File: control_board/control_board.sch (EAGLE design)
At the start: 86 parts

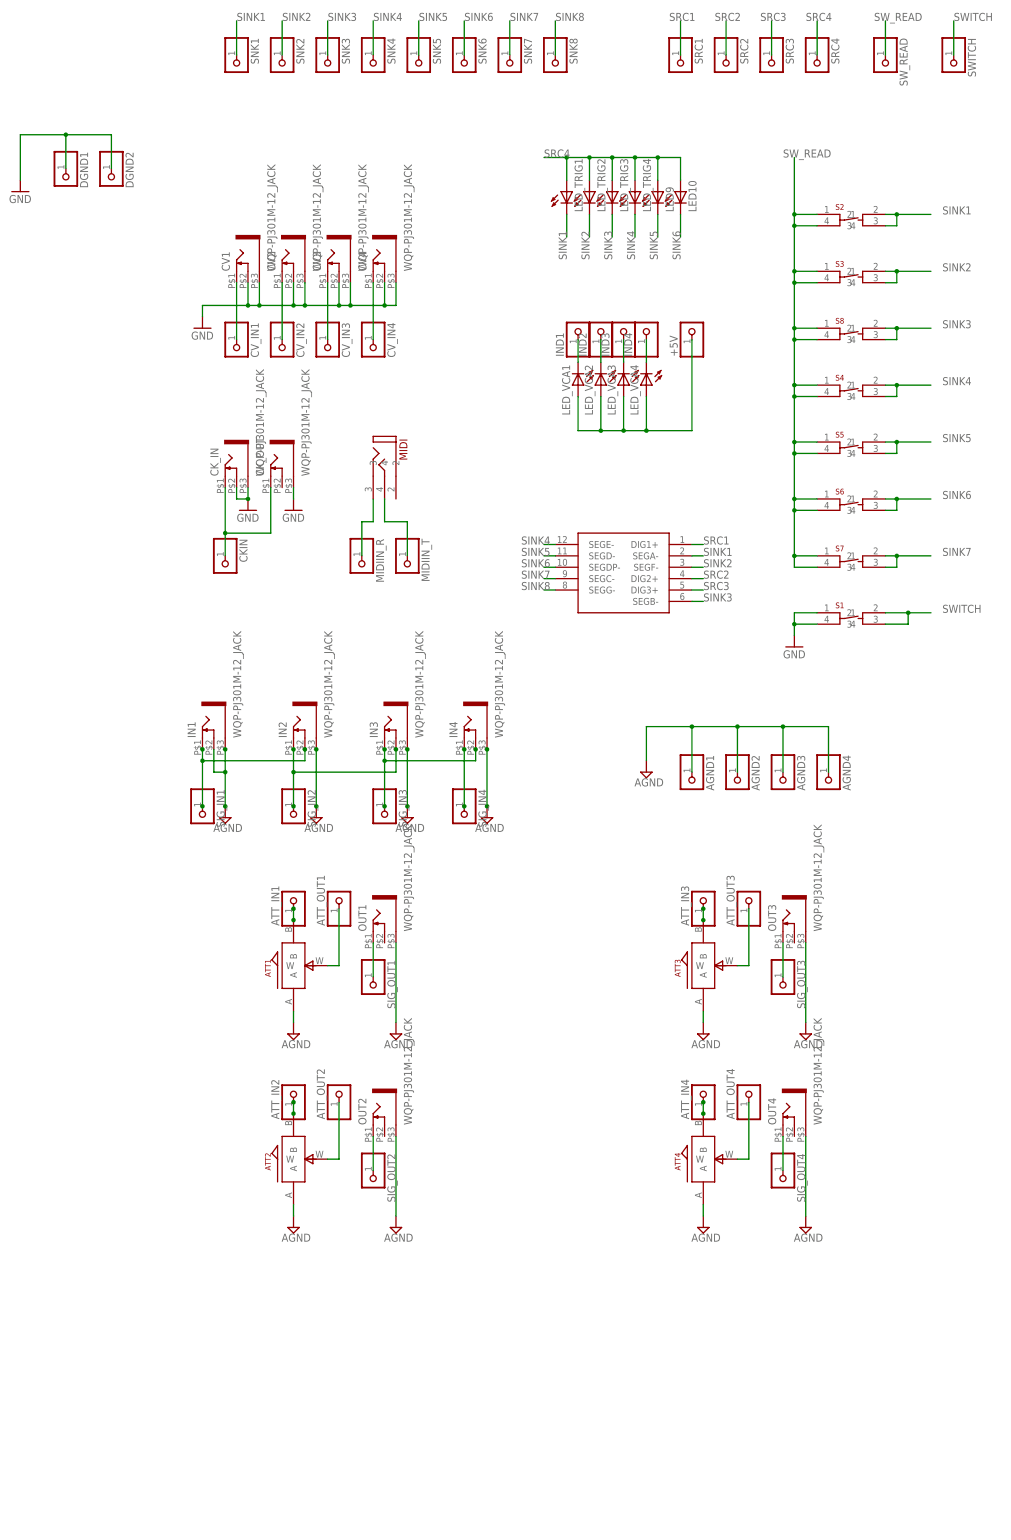
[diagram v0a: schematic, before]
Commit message: more
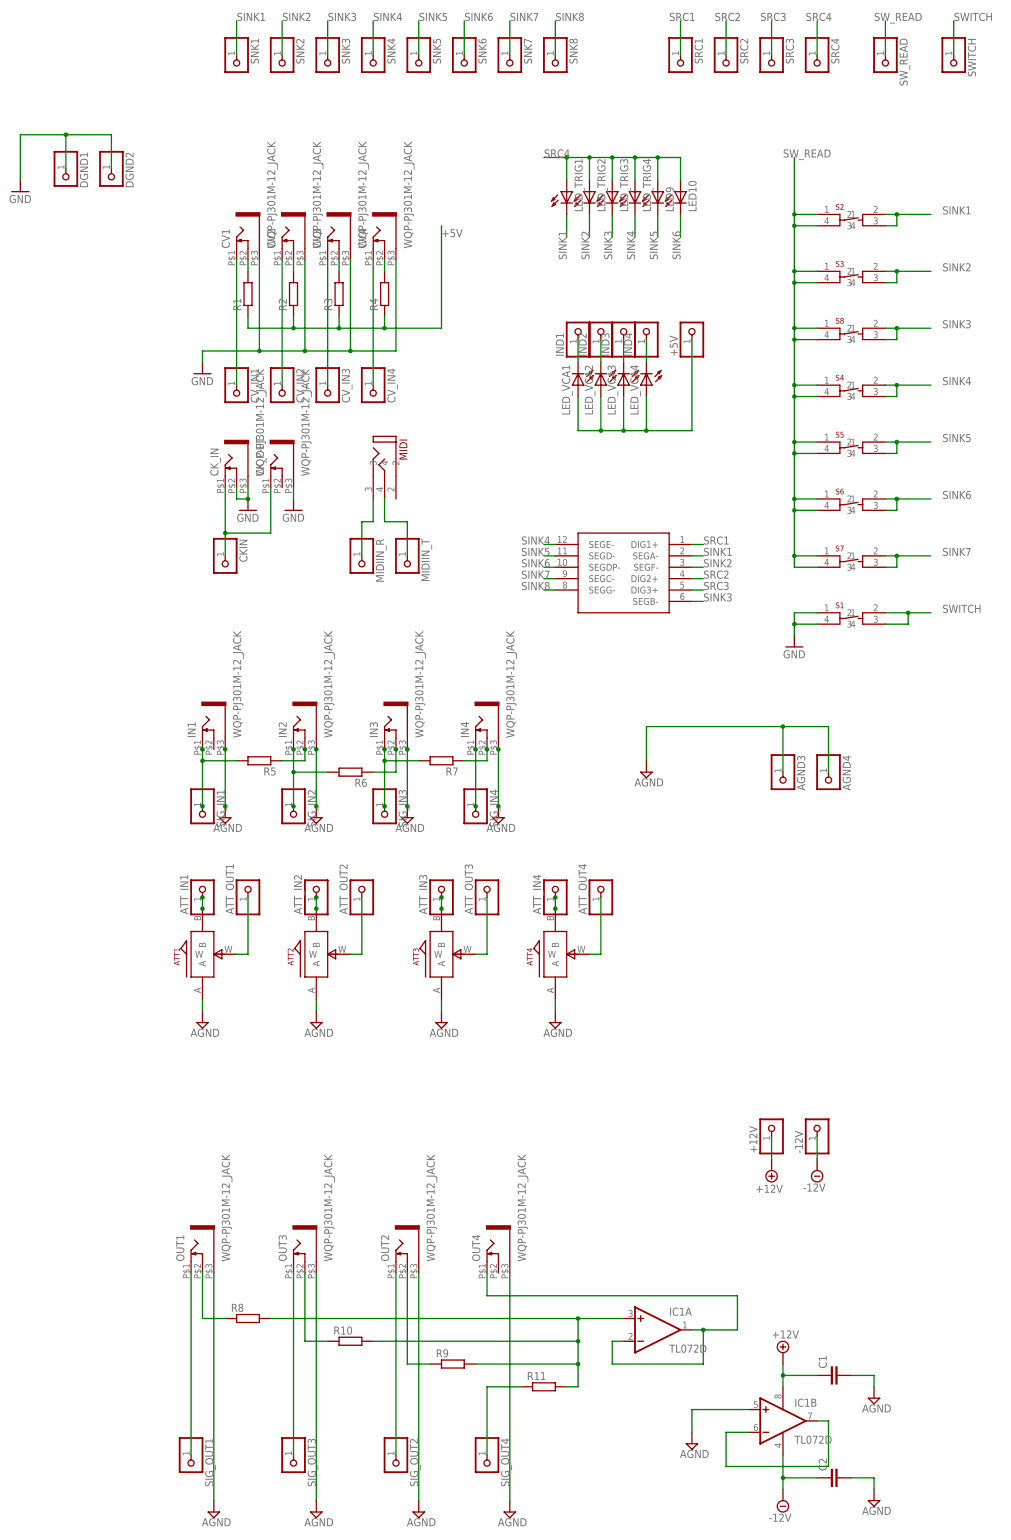
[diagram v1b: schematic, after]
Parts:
- removed AGND1, AGND2: (no value), pinhead:PINHD-1X1
- added +12V, -12V: (no value), pinhead:PINHD-1X1
- added C1, C2: (no value), rcl:C-EUC0805
- added IC1: TL072D, linear:TL072D
- added R1, R10, R11, R2, R3, R4, R5, R6, R7, R8, R9: (no value), rcl:R-EU_R0805
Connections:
- removed net N$25: +5V.1, LED_VCA1.A, LED_VCA2.A, LED_VCA3.A, LED_VCA4.A
- new net +12V: +12V.1, C1.1, IC1P.V+
- new net +5V: +5V.1, LED_VCA1.A, LED_VCA2.A, LED_VCA3.A, LED_VCA4.A, R1.1, R2.1, R3.1, R4.1
- new net -12V: -12V.1, C2.1, IC1P.V-
- new net N$29: CV1.3, R1.2
- new net N$30: CV2.3, R2.2
- new net N$31: CV3.3, R3.2
- new net N$32: CV4.3, R4.2
- new net N$34: IN2.3, R5.1
- new net N$35: IN3.3, R6.1
- new net N$36: IN4.3, R7.1
- new net N$37: IN1.2, R5.2, SIG_IN1.1
- new net N$38: OUT3.3, R10.1
- new net N$39: OUT2.3, R9.1
- new net N$42: IC1A.+IN, R10.2, R11.2, R8.2, R9.2
- new net N$44: IC1A.-IN, IC1A.OUT, OUT4.2
- new net N$46: IC1B.-IN, IC1B.OUT
- net AGND: now also C1.2, C2.2, IC1B.+IN; no longer AGND1.1, AGND2.1, IN1.3
- net GND: no longer CV1.3, CV2.3, CV3.3, CV4.3
- net N$10: now also R6.2; no longer IN3.3
- net N$11: now also R7.2; no longer IN4.3
- net N$28: now also R11.1; no longer OUT4.2
- net N$9: now also OUT1.3, R8.1; no longer IN1.2, IN2.3, SIG_IN1.1
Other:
- moved on the sheet: ATT1, ATT2, ATT3, ATT4, ATT_IN1, ATT_IN2, ATT_IN3, ATT_IN4, ATT_OUT1, ATT_OUT2, ATT_OUT3, ATT_OUT4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
